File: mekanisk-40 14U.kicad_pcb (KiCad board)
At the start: 2 copper layers, 266.7 x 76.2 mm, 148 parts, among them J2 USB_C_Receptacle_USB2.0, Q1 2N7002, SW1 RST, U1 USBLC6-2SC6, U2 XC6206PxxxMR-Regulator_Linear, U3 STM32F072C8Tx

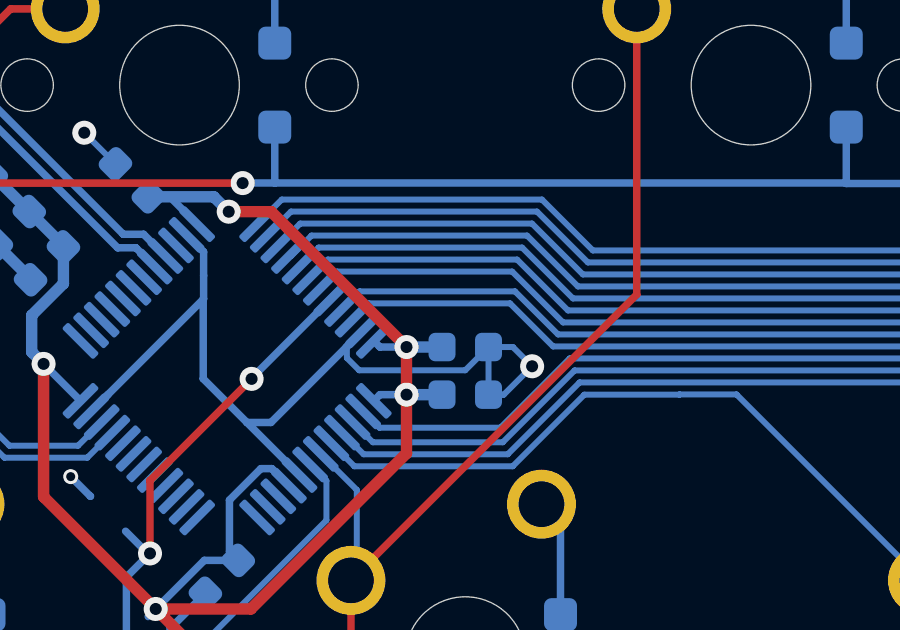
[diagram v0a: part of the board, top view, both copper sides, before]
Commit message: update
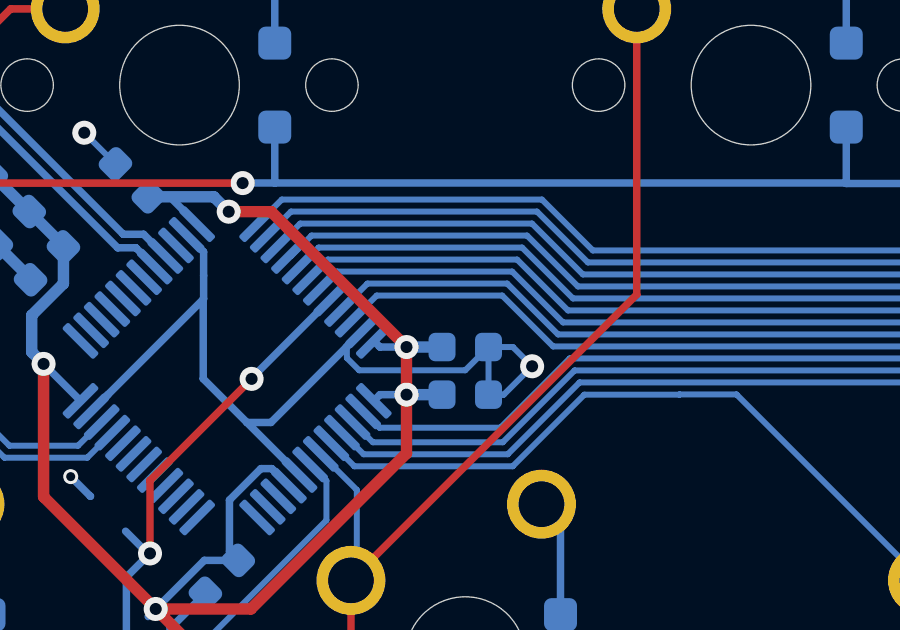
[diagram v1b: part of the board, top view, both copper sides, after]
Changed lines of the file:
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@@
     (fp_arc (start 8.53125 -5.499999) (mid 8.677685 -5.853565) (end 9.03125 -5.999999)
       (stroke (width 0.05) (type solid)) (layer "Eco2.User"))
-    (fp_arc (start 9.03125 8.000001) (mid 8.677729 7.853537) (end 8.53125 7.500001)
+    (fp_arc (start 9.03125 8.000001) (mid 8.677693 7.853543) (end 8.53125 7.500001)
       (stroke (width 0.05) (type solid)) (layer "Eco2.User"))
-    (fp_arc (start 14.780039 -5.999999) (mid 15.133567 -5.853539) (end 15.280039 -5.499999)
+    (fp_arc (start 14.780039 -5.999999) (mid 15.133602 -5.853545) (end 15.280039 -5.499999)
       (stroke (width 0.05) (type solid)) (layer "Eco2.User"))
-    (fp_arc (start 15.28125 7.500001) (mid 15.134806 7.853571) (end 14.78125 8.000001)
+    (fp_arc (start 15.28125 7.500001) (mid 15.1348 7.853536) (end 14.78125 8.000001)
       (stroke (width 0.05) (type solid)) (layer "Eco2.User"))
     (pad "" thru_hole circle (at -11.90625 -6.985) (size 4 4) (drill 3.048) (layers "*.Cu" "B.Mask"))
@@
     (fp_arc (start 8.53125 -5.499999) (mid 8.677685 -5.853565) (end 9.03125 -5.999999)
       (stroke (width 0.05) (type solid)) (layer "Eco2.User"))
-    (fp_arc (start 9.03125 8.000001) (mid 8.677729 7.853537) (end 8.53125 7.500001)
+    (fp_arc (start 9.03125 8.000001) (mid 8.677693 7.853543) (end 8.53125 7.500001)
       (stroke (width 0.05) (type solid)) (layer "Eco2.User"))
-    (fp_arc (start 14.780039 -5.999999) (mid 15.133567 -5.853539) (end 15.280039 -5.499999)
+    (fp_arc (start 14.780039 -5.999999) (mid 15.133602 -5.853545) (end 15.280039 -5.499999)
       (stroke (width 0.05) (type solid)) (layer "Eco2.User"))
-    (fp_arc (start 15.28125 7.500001) (mid 15.134806 7.853571) (end 14.78125 8.000001)
+    (fp_arc (start 15.28125 7.500001) (mid 15.1348 7.853536) (end 14.78125 8.000001)
       (stroke (width 0.05) (type solid)) (layer "Eco2.User"))
     (pad "" thru_hole circle (at -11.90625 -6.985) (size 4 4) (drill 3.048) (layers "*.Cu" "B.Mask"))
@@
     (fp_arc (start 8.53125 -5.499999) (mid 8.677685 -5.853565) (end 9.03125 -5.999999)
       (stroke (width 0.05) (type solid)) (layer "Eco2.User"))
-    (fp_arc (start 9.03125 8.000001) (mid 8.677729 7.853537) (end 8.53125 7.500001)
+    (fp_arc (start 9.03125 8.000001) (mid 8.677693 7.853543) (end 8.53125 7.500001)
       (stroke (width 0.05) (type solid)) (layer "Eco2.User"))
-    (fp_arc (start 14.780039 -5.999999) (mid 15.133567 -5.853539) (end 15.280039 -5.499999)
+    (fp_arc (start 14.780039 -5.999999) (mid 15.133602 -5.853545) (end 15.280039 -5.499999)
       (stroke (width 0.05) (type solid)) (layer "Eco2.User"))
-    (fp_arc (start 15.28125 7.500001) (mid 15.134806 7.853571) (end 14.78125 8.000001)
+    (fp_arc (start 15.28125 7.500001) (mid 15.1348 7.853536) (end 14.78125 8.000001)
       (stroke (width 0.05) (type solid)) (layer "Eco2.User"))
     (pad "" thru_hole circle (at -11.90625 -6.985 180) (size 4 4) (drill 3.048) (layers "*.Cu" "B.Mask"))
@@
     (fp_arc (start 8.53125 -5.499999) (mid 8.677685 -5.853565) (end 9.03125 -5.999999)
       (stroke (width 0.05) (type solid)) (layer "Eco2.User"))
-    (fp_arc (start 9.03125 8.000001) (mid 8.677729 7.853537) (end 8.53125 7.500001)
+    (fp_arc (start 9.03125 8.000001) (mid 8.677693 7.853543) (end 8.53125 7.500001)
       (stroke (width 0.05) (type solid)) (layer "Eco2.User"))
-    (fp_arc (start 14.780039 -5.999999) (mid 15.133567 -5.853539) (end 15.280039 -5.499999)
+    (fp_arc (start 14.780039 -5.999999) (mid 15.133602 -5.853545) (end 15.280039 -5.499999)
       (stroke (width 0.05) (type solid)) (layer "Eco2.User"))
-    (fp_arc (start 15.28125 7.500001) (mid 15.134806 7.853571) (end 14.78125 8.000001)
+    (fp_arc (start 15.28125 7.500001) (mid 15.1348 7.853536) (end 14.78125 8.000001)
       (stroke (width 0.05) (type solid)) (layer "Eco2.User"))
     (pad "" thru_hole circle (at -11.90625 -6.985 180) (size 4 4) (drill 3.048) (layers "*.Cu" "B.Mask"))
@@
     (fp_arc (start 8.53125 -5.499999) (mid 8.677685 -5.853565) (end 9.03125 -5.999999)
       (stroke (width 0.05) (type solid)) (layer "Eco2.User"))
-    (fp_arc (start 9.03125 8.000001) (mid 8.677729 7.853537) (end 8.53125 7.500001)
+    (fp_arc (start 9.03125 8.000001) (mid 8.677693 7.853543) (end 8.53125 7.500001)
       (stroke (width 0.05) (type solid)) (layer "Eco2.User"))
-    (fp_arc (start 14.780039 -5.999999) (mid 15.133567 -5.853539) (end 15.280039 -5.499999)
+    (fp_arc (start 14.780039 -5.999999) (mid 15.133602 -5.853545) (end 15.280039 -5.499999)
       (stroke (width 0.05) (type solid)) (layer "Eco2.User"))
-    (fp_arc (start 15.28125 7.500001) (mid 15.134806 7.853571) (end 14.78125 8.000001)
+    (fp_arc (start 15.28125 7.500001) (mid 15.1348 7.853536) (end 14.78125 8.000001)
       (stroke (width 0.05) (type solid)) (layer "Eco2.User"))
     (pad "" thru_hole circle (at -11.90625 -6.985) (size 4 4) (drill 3.048) (layers "*.Cu" "B.Mask"))
@@
   (segment (start 163.98875 38.735) (end 163.98875 53.0225) (width 0.25) (layer "F.Cu") (net 57))
   (segment (start 168.75125 57.785) (end 168.75125 67.31) (width 0.25) (layer "F.Cu") (net 57))
-  (segment (start 70.713034 69.0361) (end 69.278102 67.601167) (width 0.2) (layer "B.Cu") (net 57))
-  (segment (start 69.278102 67.601167) (end 64.572457 67.601167) (width 0.2) (layer "B.Cu") (net 57))
-  (segment (start 64.572457 67.601167) (end 64.029519 68.144105) (width 0.2) (layer "B.Cu") (net 57))
-  (segment (start 151.42735 69.0361) (end 70.713034 69.0361) (width 0.2) (layer "B.Cu") (net 57))
+  (segment (start 69.017441 67.340507) (end 64.833117 67.340507) (width 0.2) (layer "B.Cu") (net 57))
+  (segment (start 64.833117 67.340507) (end 64.029519 68.144105) (width 0.2) (layer "B.Cu") (net 57))
+  (segment (start 70.713034 69.0361) (end 69.017441 67.340507) (width 0.2) (layer "B.Cu") (net 57))
   (segment (start 159.22625 76.835) (end 151.42735 69.0361) (width 0.2) (layer "B.Cu") (net 57))
+  (segment (start 151.42735 69.0361) (end 70.713034 69.0361) (width 0.2) (layer "B.Cu") (net 57))
   (segment (start 187.80125 57.785) (end 187.80125 67.31) (width 0.25) (layer "F.Cu") (net 58))
   (segment (start 183.03875 38.735) (end 183.03875 53.0225) (width 0.25) (layer "F.Cu") (net 58))
   (segment (start 183.03875 53.0225) (end 187.80125 57.785) (width 0.25) (layer "F.Cu") (net 58))
   (segment (start 187.80125 67.31) (end 178.27625 76.835) (width 0.25) (layer "F.Cu") (net 58))
-  (segment (start 69.443787 67.201167) (end 64.265349 67.201167) (width 0.2) (layer "B.Cu") (net 58))
-  (segment (start 64.265349 67.201167) (end 63.675965 67.790551) (width 0.2) (layer "B.Cu") (net 58))
-  (segment (start 70.87872 68.6361) (end 69.443787 67.201167) (width 0.2) (layer "B.Cu") (net 58))
-  (segment (start 178.27625 76.835) (end 170.07735 68.6361) (width 0.2) (layer "B.Cu") (net 58))
+  (segment (start 64.526009 66.940507) (end 63.675965 67.790551) (width 0.2) (layer "B.Cu") (net 58))
+  (segment (start 69.183127 66.940507) (end 64.526009 66.940507) (width 0.2) (layer "B.Cu") (net 58))
   (segment (start 170.07735 68.6361) (end 70.87872 68.6361) (width 0.2) (layer "B.Cu") (net 58))
+  (segment (start 70.87872 68.6361) (end 69.183127 66.940507) (width 0.2) (layer "B.Cu") (net 58))
+  (segment (start 178.27625 76.835) (end 170.07735 68.6361) (width 0.2) (layer "B.Cu") (net 58))
   (segment (start 206.85125 57.785) (end 206.85125 67.31) (width 0.25) (layer "F.Cu") (net 59))
   (segment (start 206.85125 67.31) (end 197.32625 76.835) (width 0.25) (layer "F.Cu") (net 59))
